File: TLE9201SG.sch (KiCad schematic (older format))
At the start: 6 parts, among them U4 TLE9201SG

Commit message: manual sync with 960
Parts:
- C19: Manufacturer WURTH -> (none); Part # 885012208052 -> (none); VEND MOUSER -> (none); VEND# 710-885012208052 -> (none)
- U4: Part # (none) -> 726-TLE9201SG
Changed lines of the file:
@@
 F 2 "Capacitor_SMD:C_0603_1608Metric_Pad1.05x0.95mm_HandSolder" H 7400 4000 50  0001 C CNN
 F 3 "~" H 7400 4000 50  0001 C CNN
-F 4 "WURTH" H 1800 450 50  0001 C CNN "Manufacturer"
-F 5 "885012208052" H 1800 450 50  0001 C CNN "Part #"
-F 6 "MOUSER" H 1800 450 50  0001 C CNN "VEND"
-F 7 "710-885012208052" H 1800 450 50  0001 C CNN "VEND#"
 	1    7400 4000
 	1    0    0    -1
@@
 F 2 "Package_SO:Infineon_PG-DSO-12-11" H 5525 3100 50  0001 C CNN
 F 3 "" H 5525 3100 50  0001 C CNN
+F 4 "726-TLE9201SG" H 0   0   50  0001 C CNN "Part #"
 	1    5525 3100
 	1    0    0    -1

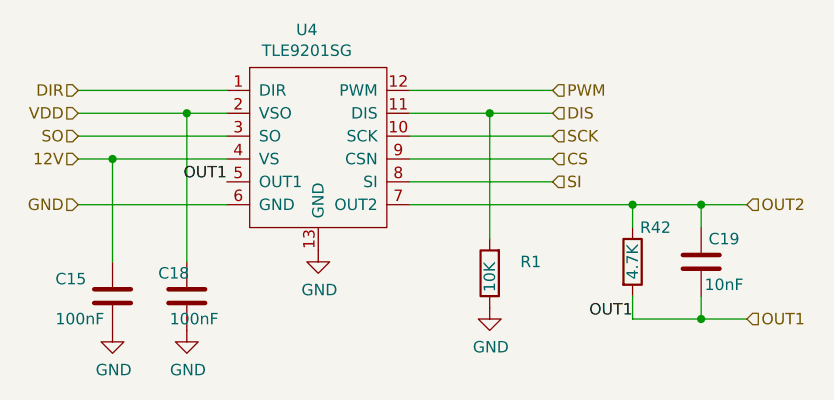
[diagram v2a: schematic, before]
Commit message: Update (#46)
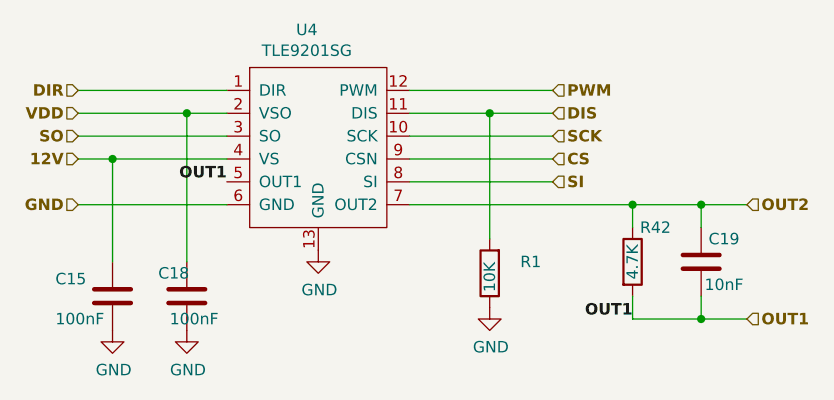
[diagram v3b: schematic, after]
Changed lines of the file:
@@
 Comment4 ""
 $EndDescr
-Text HLabel 7600 3750 2    50   Input ~ 0
+Text HLabel 7600 3750 2    50   Input ~ 6
 OUT2
-Text HLabel 7600 4250 2    50   Input ~ 0
+Text HLabel 7600 4250 2    50   Input ~ 6
 OUT1
-Text HLabel 4675 3550 0    50   Input ~ 0
+Text HLabel 4675 3550 0    50   Input ~ 6
 12V
-Text HLabel 4675 3350 0    50   Input ~ 0
+Text HLabel 4675 3350 0    50   Input ~ 6
 VDD
-Text HLabel 4675 3250 0    50   Input ~ 0
+Text HLabel 4675 3250 0    50   Input ~ 6
 DIR
-Text HLabel 4675 3450 0    50   Input ~ 0
+Text HLabel 4675 3450 0    50   Input ~ 6
 SO
-Text HLabel 6750 3250 2    50   Input ~ 0
+Text HLabel 6750 3250 2    50   Input ~ 6
 PWM
-Text HLabel 6750 3350 2    50   Input ~ 0
+Text HLabel 6750 3350 2    50   Input ~ 6
 DIS
-Text HLabel 6750 3450 2    50   Input ~ 0
+Text HLabel 6750 3450 2    50   Input ~ 6
 SCK
-Text HLabel 6750 3550 2    50   Input ~ 0
+Text HLabel 6750 3550 2    50   Input ~ 6
 CS
-Text HLabel 6750 3650 2    50   Input ~ 0
+Text HLabel 6750 3650 2    50   Input ~ 6
 SI
-Text HLabel 4675 3750 0    50   Input ~ 0
+Text HLabel 4675 3750 0    50   Input ~ 6
 GND
 Wire Wire Line
@@
 Wire Wire Line
 	6125 3750 7100 3750
-Text Label 5325 3650 2    50   ~ 0
+Text Label 5325 3650 2    50   ~ 6
 OUT1
-Text Label 7100 4250 2    50   ~ 0
+Text Label 7100 4250 2    50   ~ 6
 OUT1
 Connection ~ 5150 3350
